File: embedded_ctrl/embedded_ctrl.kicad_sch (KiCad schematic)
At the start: 19 parts, among them J1 Conn_02x13_Odd_Even, J2 DB25_Plug, J3 Conn_01x15_Socket, J4 Conn_01x15_Socket, J5 Conn_01x06, J6 Screw_Terminal_01x02, J7 USB_B, J8 Conn_01x02_Pin

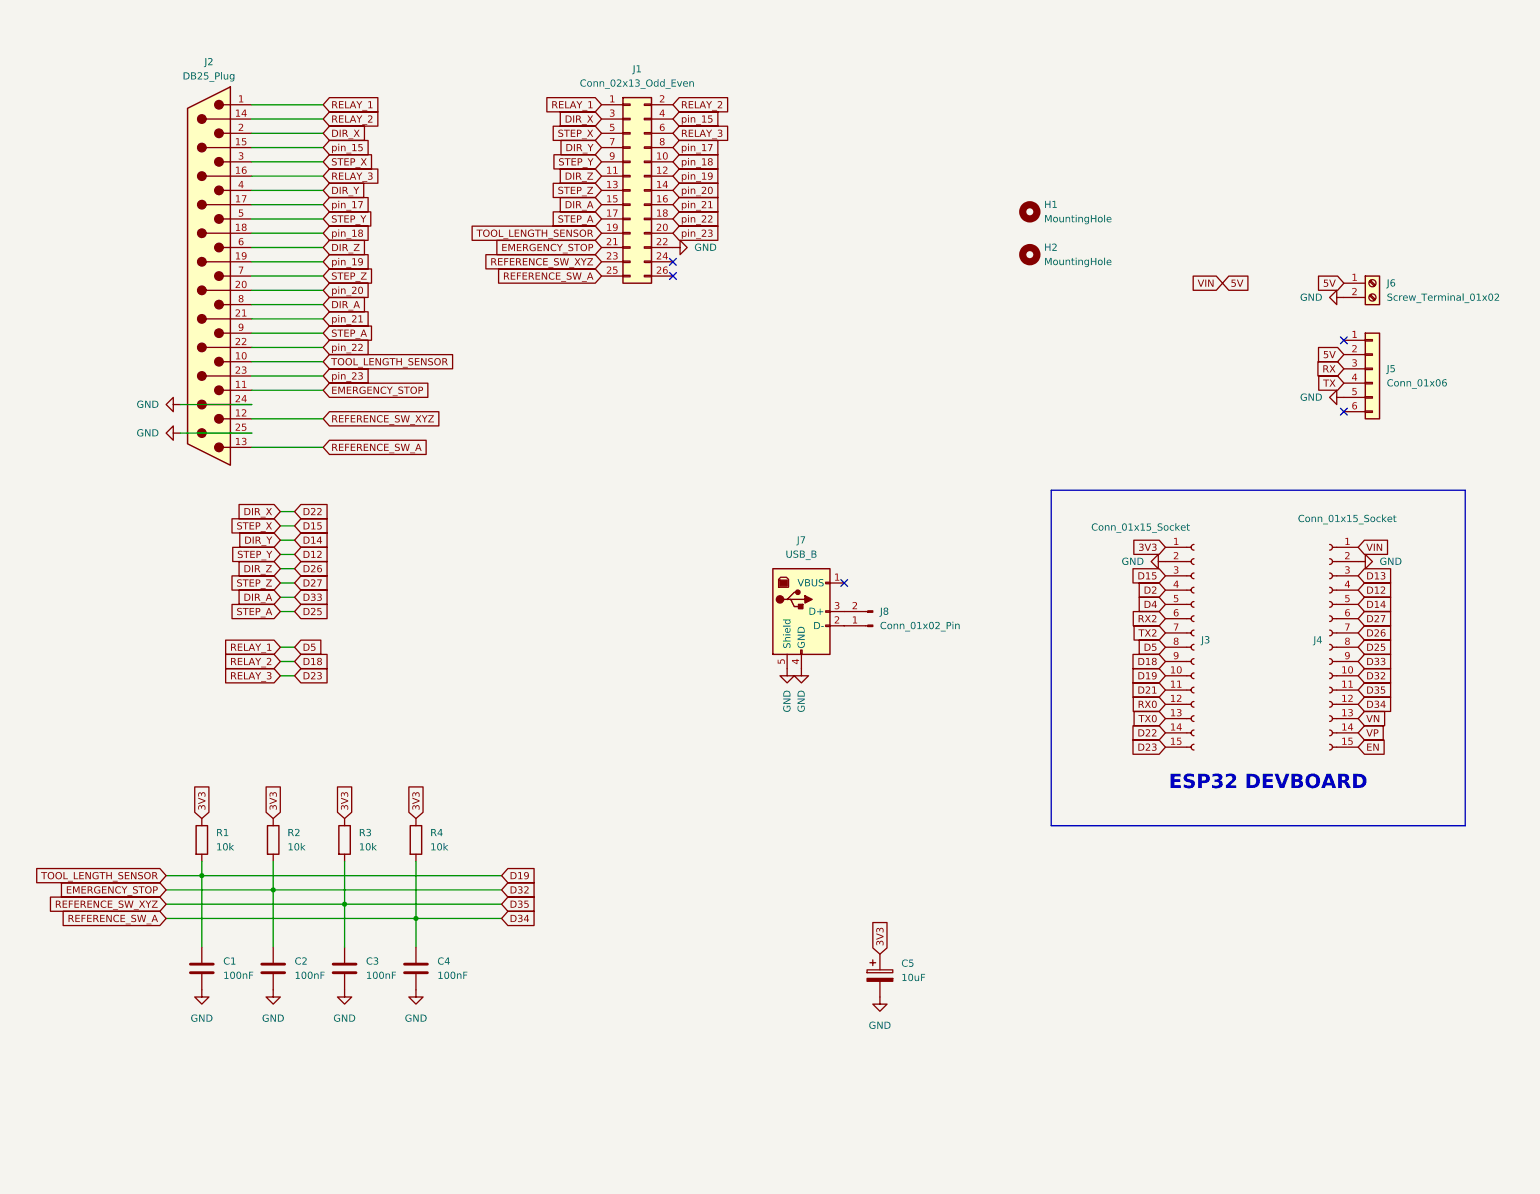
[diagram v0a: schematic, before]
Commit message: more work on embedded ctrlr
same-o
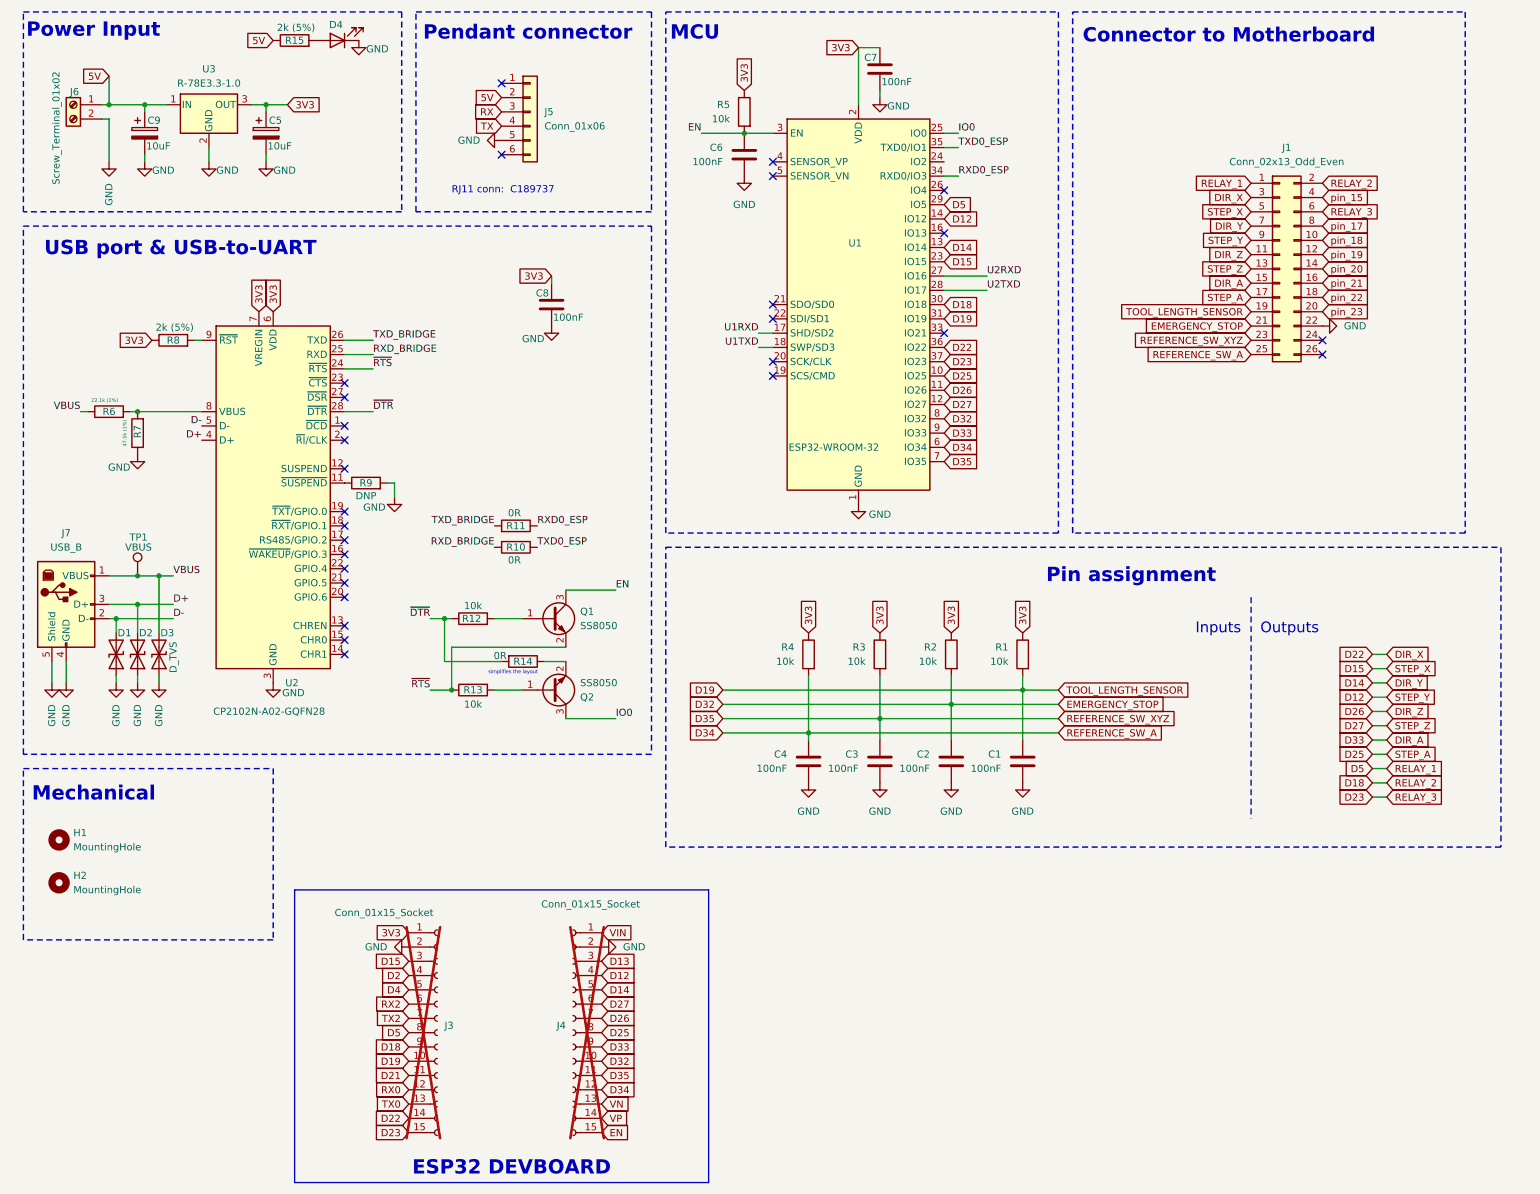
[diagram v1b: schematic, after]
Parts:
- removed J2: DB25_Plug, Connector_Dsub:DSUB-25_Male_Horizontal_P2.77x2.54mm_EdgePinOffset9.40mm, symbol Connector:DB25_Plug
- removed J8: Conn_01x02_Pin, symbol Connector:Conn_01x02_Pin
- added C6, C7, C8: 100nF, Capacitor_SMD:C_0603_1608Metric, symbol Device:C
- added C9: 10uF, Capacitor_SMD:CP_Elec_5x5.4, symbol Device:C_Polarized
- added D1, D2, D3: D_TVS, Diode_SMD:D_0603_1608Metric, symbol Device:D_TVS
- added D4: LED, Diode_SMD:D_0603_1608Metric, symbol Device:LED
- added Q1, Q2: SS8050, Package_TO_SOT_SMD:SOT-23, symbol Transistor_BJT:SS8050
- added R10, R11, R14: 0R, Resistor_SMD:R_0603_1608Metric, symbol Device:R
- added R12, R13, R5: 10k, Resistor_SMD:R_0603_1608Metric, symbol Device:R
- added R15, R8: 2k (5%), Resistor_SMD:R_0603_1608Metric, symbol Device:R
- added R6: 22.1k (1%), Resistor_SMD:R_0603_1608Metric, symbol Device:R
- added R7: 47.5k (1%), Resistor_SMD:R_0603_1608Metric, symbol Device:R
- added R9: DNP, Resistor_SMD:R_0603_1608Metric, symbol Device:R
- added TP1: VBUS, symbol Connector:TestPoint
- added U1: ESP32-WROOM-32, RF_Module:ESP32-WROOM-32, symbol RF_Module:ESP32-WROOM-32
- added U2: CP2102N-A02-GQFN28, Package_DFN_QFN:QFN-28-1EP_5x5mm_P0.5mm_EP3.35x3.35mm, symbol Interface_USB:CP2102N-Axx-xQFN28
- added U3: R-78E3.3-1.0, Converter_DCDC:Converter_DCDC_RECOM_R-78E-0.5_THT, symbol Regulator_Switching:R-78E3.3-1.0
- C1, C2, C3, C4: JLCPCB Part # (none) -> C14663
- C5: footprint Capacitor_SMD:CP_Elec_5x5.8 -> Capacitor_SMD:CP_Elec_5x5.4; JLCPCB Part # (none) -> C72487
- J1: JLCPCB Part # (none) -> C2894993
- J3, J4: footprint Connector_PinSocket_2.54mm:PinSocket_1x15_P2.54mm_Vertical -> (none); now not fitted
- J6: JLCPCB Part # (none) -> C8465
- J7: footprint (none) -> Connector_USB:USB_B_OST_USB-B1HSxx_Horizontal; JLCPCB Part # (none) -> C720549
- R1, R2, R3, R4: JLCPCB Part # (none) -> C25804
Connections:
- net 3V3: now also C7.1, C8.1, R5.1, R8.1, U1.2 (VDD), U2.6 (VDD), U2.7 (VREGIN), U3.3 (OUT)
- net 5V: now also C9.1, R15.1, U3.1 (IN); no longer J4.1 (Pin_1)
- net D12: now also U1.14 (IO12)
- net D14: now also U1.13 (IO14)
- net D15: now also U1.23 (IO15)
- net D18: now also U1.30 (IO18)
- net D19: now also U1.31 (IO19)
- net D22: now also U1.36 (IO22)
- net D23: now also U1.37 (IO23)
- net D25: now also U1.10 (IO25)
- net D26: now also U1.11 (IO26)
- net D27: now also U1.12 (IO27)
- net D32: now also U1.8 (IO32)
- net D33: now also U1.9 (IO33)
- net D34: now also U1.6 (IO34)
- net D35: now also U1.7 (IO35)
- net D5: now also U1.29 (IO5)
- net EN: now also C6.1, Q1.3 (C), R5.2, U1.3 (EN)
- net GND: now also C6.2, C7.2, C8.2, C9.2, D1.1 (A1), D2.1 (A1), D3.1 (A1), D4.1 (K), R7.1, R9.2, U1.1 (GND), U1.15 (GND), U1.38 (GND), U1.39 (GND), U2.29 (GND), U2.3 (GND), U3.2 (GND)
- net D-: now reaches J7.2 (D-)
- net D-: now also D1.2 (A2), U2.5 (D-)
- net D+: now reaches J7.3 (D+)
- net D+: now also D2.2 (A2), U2.4 (D+)
- net VBUS: now reaches J7.1 (VBUS)
- net VBUS: now also D3.2 (A2), R6.1, TP1.1
- new net: R6.2, R7.2, U2.8 (VBUS)
- new net: Q1.1 (B), R12.2
- new net: D4.2 (A), R15.2
- new net: R9.1, U2.11 (~{SUSPEND})
- new net: R8.2, U2.9 (~{RST})
- new net: Q2.2 (E), R14.1
- new net: Q2.1 (B), R13.2
- new net IO0: Q2.3 (C), U1.25 (IO0)
- new net RXD0_ESP: R11.1, U1.34 (RXD0/IO3)
- new net RXD_BRIDGE: R10.2, U2.25 (RXD)
- new net TXD0_ESP: R10.1, U1.35 (TXD0/IO1)
- new net TXD_BRIDGE: R11.2, U2.26 (TXD)
- new net U1RXD: U1.17 (SHD/SD2)
- new net U1TXD: U1.18 (SWP/SD3)
- new net U2RXD: U1.27 (IO16)
- new net U2TXD: U1.28 (IO17)
- new net VIN: J4.1 (Pin_1)
- new net ~{DTR}: R12.1, R14.2, U2.28 (~{DTR})
- new net ~{RTS}: Q1.2 (E), R13.1, U2.24 (~{RTS})
- no-connect marks 5 -> 28
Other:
- note added: "Connector to Motherboard"
- note added: "Inputs"
- note added: "MCU"
- note added: "Mechanical"
- note added: "Outputs"
- note added: "Pendant connector"
- note added: "Pin assignment"
- note added: "Power Input"
- note added: "RJ11 conn: C189737"
- note added: "USB port & USB-to-UART"
- note added: "simplifies the layout"
- moved on the sheet: C1, C2, C3, C4, C5, H1, H2, J1, J5, J6, J7, R1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
